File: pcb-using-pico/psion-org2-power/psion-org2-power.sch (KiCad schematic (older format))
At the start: 14 parts, among them J1 Conn_02x08_Odd_Even, J2 Conn_02x08_Odd_Even, J3 Conn_01x27_Female, J4 Conn_02x08_Odd_Even, U6 74LS245, U7 74LS245

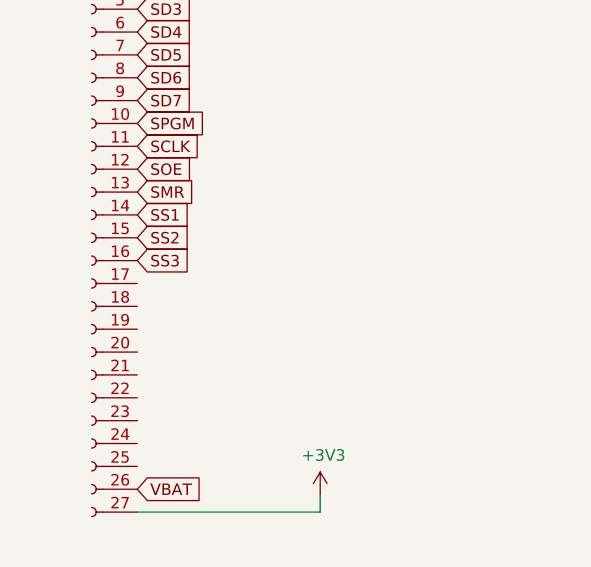
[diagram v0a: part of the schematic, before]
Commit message: Updates to both PCBs
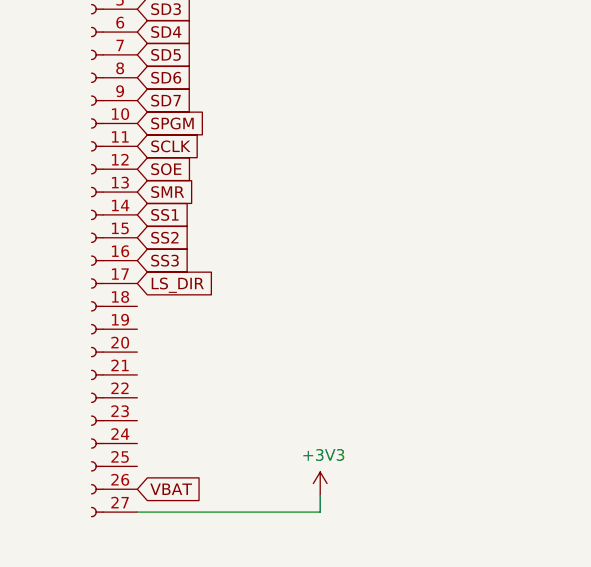
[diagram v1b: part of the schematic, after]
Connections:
- net LS_DIR: now also J3.17 (Pin_17)
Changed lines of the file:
@@
 Wire Wire Line
 	11175 6225 10650 6225
+Text GLabel 1950 8175 2    50   Input ~ 0
+LS_DIR
 $EndSCHEMATC
